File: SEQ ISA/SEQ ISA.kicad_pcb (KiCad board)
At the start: 2 copper layers, 70 x 65 mm, 70 parts, among them IC1 TLX9310_TPL,F, IC2 SN74LVC4245ADW, J1 FTSH-107-01-L-DV-K-A, J2 Conn_01x02_Pin, J3 Conn_01x02_Pin, J4 Conn_01x02_Pin, J5 Conn_01x02_Pin, J6 Conn_01x02_Pin, J7 Jack-DC, J8 Conn_01x04_Pin, M4 SERVO-MOTOR, M5 SERVO-MOTOR, M6 SERVO-MOTOR, Q1 BS170F, SW1 PRISE JACK, SW2 SW_SPDT, SW3 INTER_ACT, SW4 BP1, SW5 BP1, SW6 INTER_MIC, SW7 INTER_GENERAL, U1 STM32L010C6T6R, U3 LD1117S33TR_SOT223

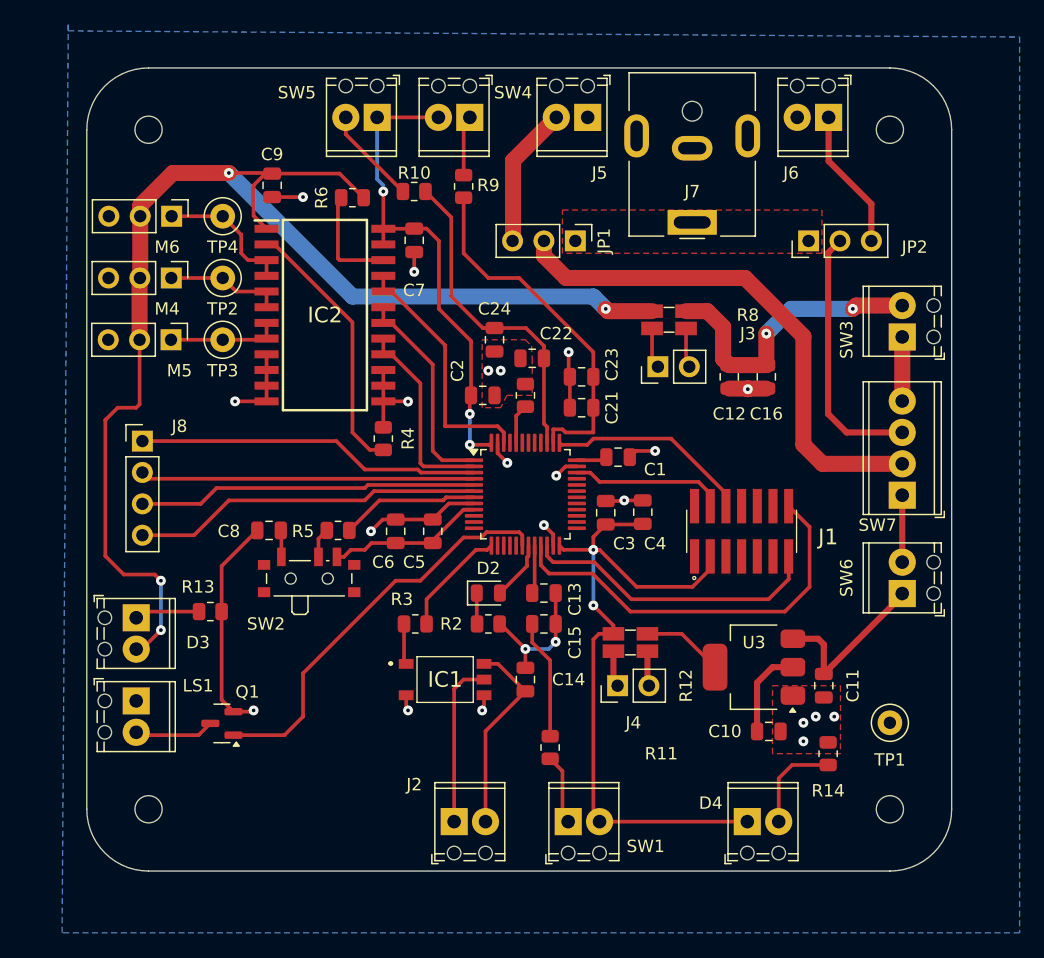
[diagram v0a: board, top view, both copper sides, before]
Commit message: Finishing PCB
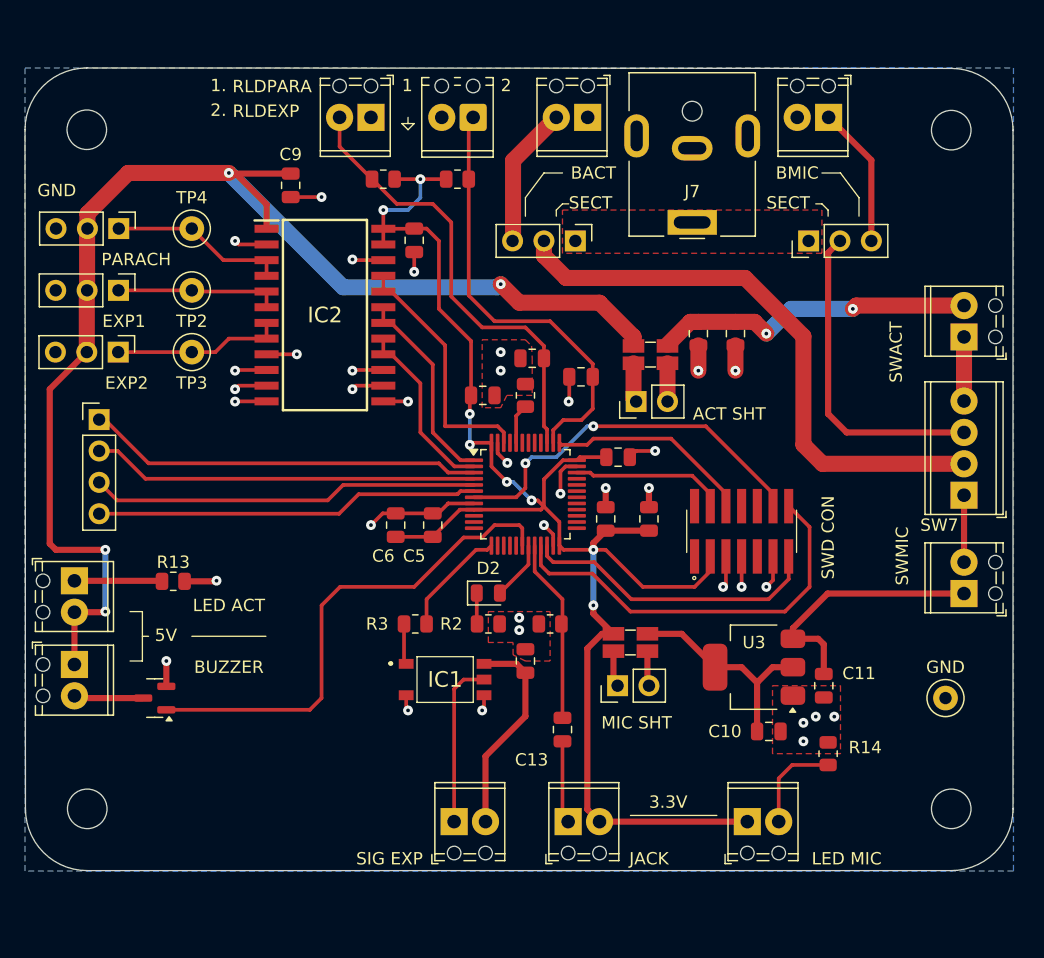
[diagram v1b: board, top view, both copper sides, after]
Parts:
- removed C15, C24, C8: 10u, Capacitor_SMD:C_0805_2012Metric
- removed C21: 100n, Capacitor_SMD:C_0805_2012Metric
- removed R4, R5, R6: 10k, Resistor_SMD:R_0805_2012Metric
- removed R9: 5.6k, Resistor_SMD:R_0805_2012Metric
- removed SW2: SW_SPDT, Button_Switch_SMD:SW_SPDT_PCM12
- removed SW4: BP1, TerminalBlock_Phoenix:TerminalBlock_Phoenix_MPT-0,5-2-2.54_1x02_P2.54mm_Horizontal
- added R15: 5.6k, Resistor_SMD:R_0805_2012Metric, F.Cu at (129.0, 53.0)
- added RLDEXP: BP1, TerminalBlock_Phoenix:TerminalBlock_Phoenix_MPT-0,5-2-2.54_1x02_P2.54mm_Horizontal, F.Cu at (130.3, 48.0)
- ACT SHT: renamed from J3
- C13, C22: value 100n -> 10n
- C23: value 10u -> 10n
- H1, H2, H3, H4: footprint MountingHole:MountingHole_2.2mm_M2 -> MountingHole:MountingHole_3.2mm_M3
- LED ACT: renamed from D3
- LED MIC: renamed from D4
- MIC SHT: renamed from J4
- R13, R14, R2: value 430 -> 1k
- RLDPARA: renamed from SW5; value BP1 -> BP2
- SIG EXP: renamed from J2
- SWD CON: renamed from J1
- moved C13 11.2 mm to (137.5, 97.5), turned to 90 degrees
- moved R11 10.0 mm to (136.5, 89.0), turned to 0 degrees
- moved LED ACT 5.83 mm to (98.0, 85.5)
- moved Q1 5.81 mm to (104.5, 95.0)
- moved BUZZER 5.81 mm to (98.0, 92.3)
- moved H1 5.00 mm to (99.0, 49.0)
- moved SW7 5.00 mm to (170.0, 78.6)
- moved SWACT 5.00 mm to (170.0, 65.8)
- moved SWMIC 5.00 mm to (170.0, 86.5)
- moved H4 4.96 mm to (99.0, 104.0)
- moved H2 4.96 mm to (169.0, 49.0)
- moved H3 4.96 mm to (169.0, 104.0)
- moved GND 4.92 mm to (168.5, 95.0)
- moved EXP1 4.39 mm to (101.6, 62.0)
- moved EXP2 4.39 mm to (101.5, 67.0)
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- renumbered J5 to BACT, J6 to BMIC, LS1 to BUZZER, M4 to EXP1, M5 to EXP2, TP1 to GND, SW1 to JACK, M6 to PARACH, J8 to PC14-15, SW3 to SWACT, SW6 to SWMIC
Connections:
- C13 pad 1: /LAUNCH_SIG -> Net-(SW1-A)
- C13 pad 2: GND -> /LAUNCH_SIG
- C23 pad 1: /RLD_EXP -> GND
- C23 pad 2: GND -> /RLD_EXP
- IC2 pad 2: Net-(IC2-DIR) -> GND
- IC2 pad 22: Net-(IC2-~{OE}) -> GND
- J7 pad 2: unconnected-(J7-Pad2) -> GND
- J7 pad MP: (no net) -> GND
- R10 pad 1: Net-(R10-Pad1) -> +3.3V
- R11 pad 1: Net-(SW1-A) -> GND
- RLDPARA pad 1: +3.3V -> GND
- RLDPARA pad 2: Net-(R10-Pad1) -> /RLD_PARA
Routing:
- net Net-(IC2-DIR): track 21.6 -> 0.00 mm
- net /NRST: track 11.2 -> 31.0 mm, vias 0 -> 2
- net +3.3V: track 112.8 -> 126.4 mm, vias 5 -> 8
- net /RLD_PARA: track 26.5 -> 37.0 mm
- net Net-(IC2-~{OE}): track 9.17 -> 0.00 mm
- net Net-(R10-Pad1): track 7.92 -> 0.00 mm
- net /BUZZER: track 33.2 -> 40.9 mm
- net GND: track 76.9 -> 69.4 mm, vias 23 -> 36
- net Net-(SW6-A): track 14.2 -> 21.0 mm
- net /RLD_EXP: track 29.3 -> 35.5 mm
- net Net-(JP1-C): track 42.3 -> 47.3 mm
- net Net-(R9-Pad1): track 4.88 -> 0.00 mm
- net Net-(JP2-C): track 21.2 -> 26.0 mm
- net /PWM2_EXP5: track 9.04 -> 13.7 mm
- net /PC14: track 27.9 -> 32.1 mm
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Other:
- board size 70 x 65 mm -> 80 x 65 mm
- board text added: "1"
- board text added: "1."
- board text added: "2"
- board text added: "2."
- board text added: "3.3V"
- board text added: "5V"
- board text added: "GND"
- board text added: "PC14"
- board text added: "PC15"
- board text added: "PH0"
- board text added: "PH1"
- board text added: "SECT"
